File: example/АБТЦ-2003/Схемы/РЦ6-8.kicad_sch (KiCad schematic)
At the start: 32 parts

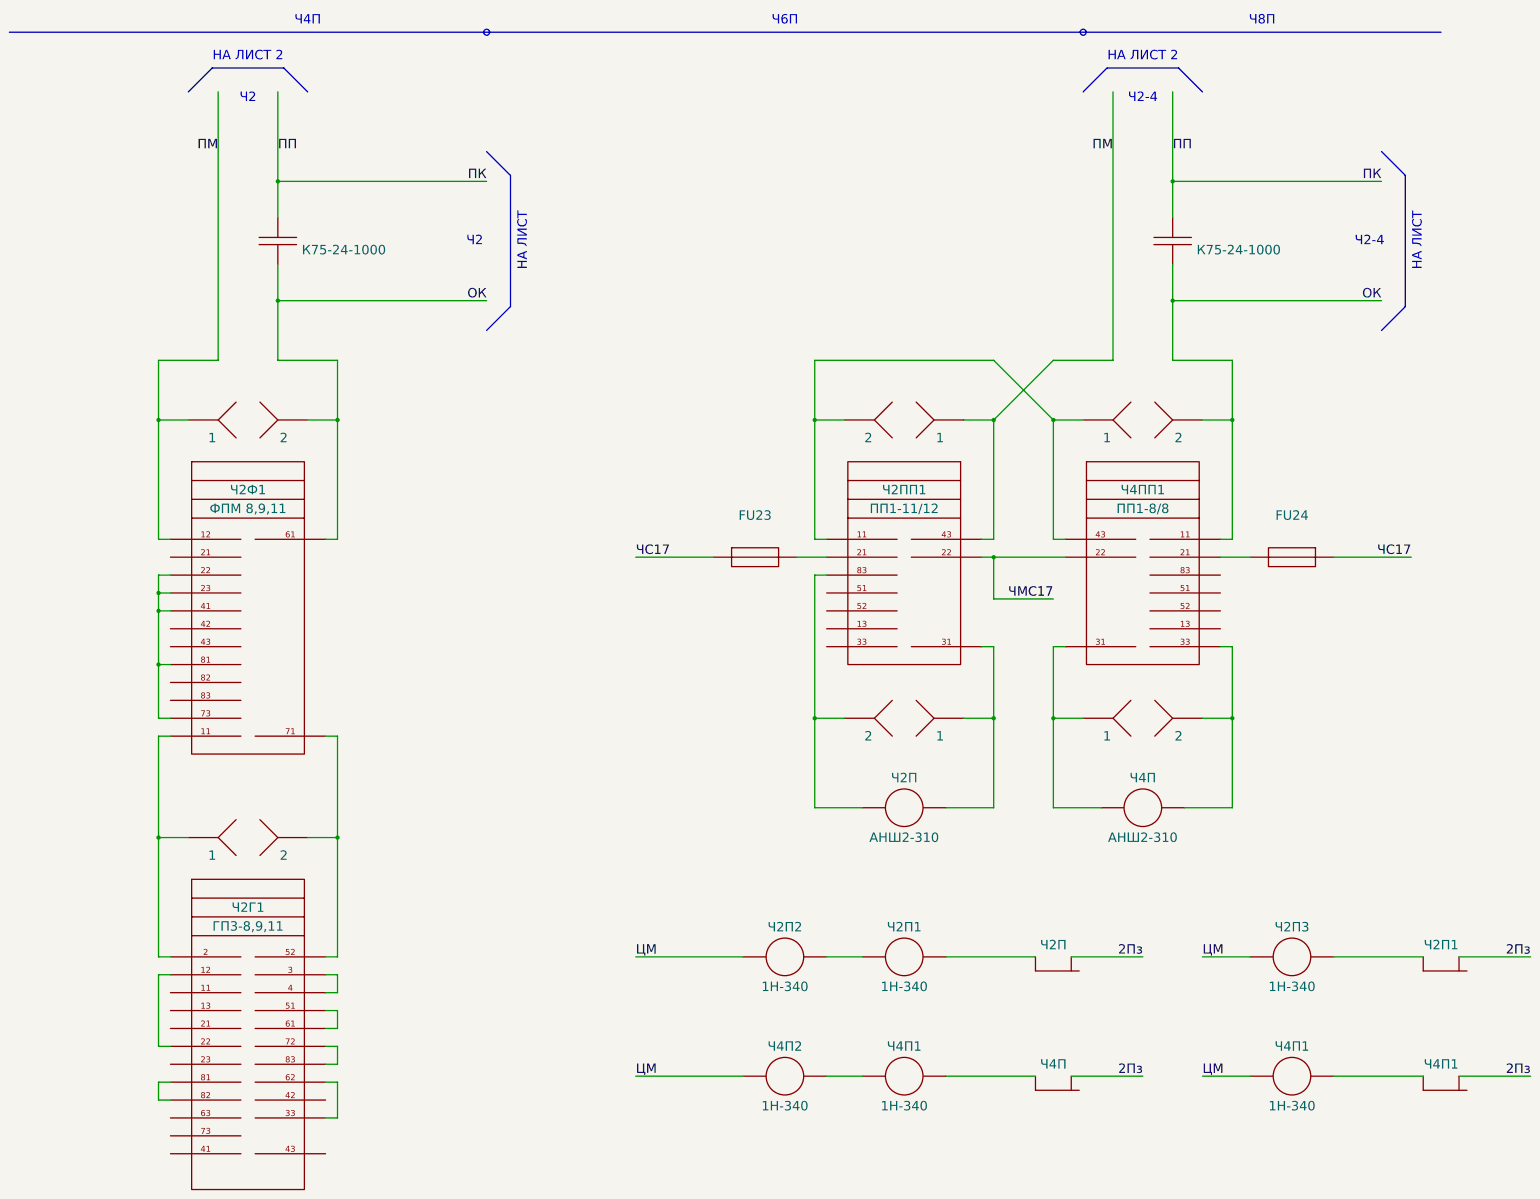
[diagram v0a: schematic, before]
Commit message: Шаблон АБТЦ обновлен
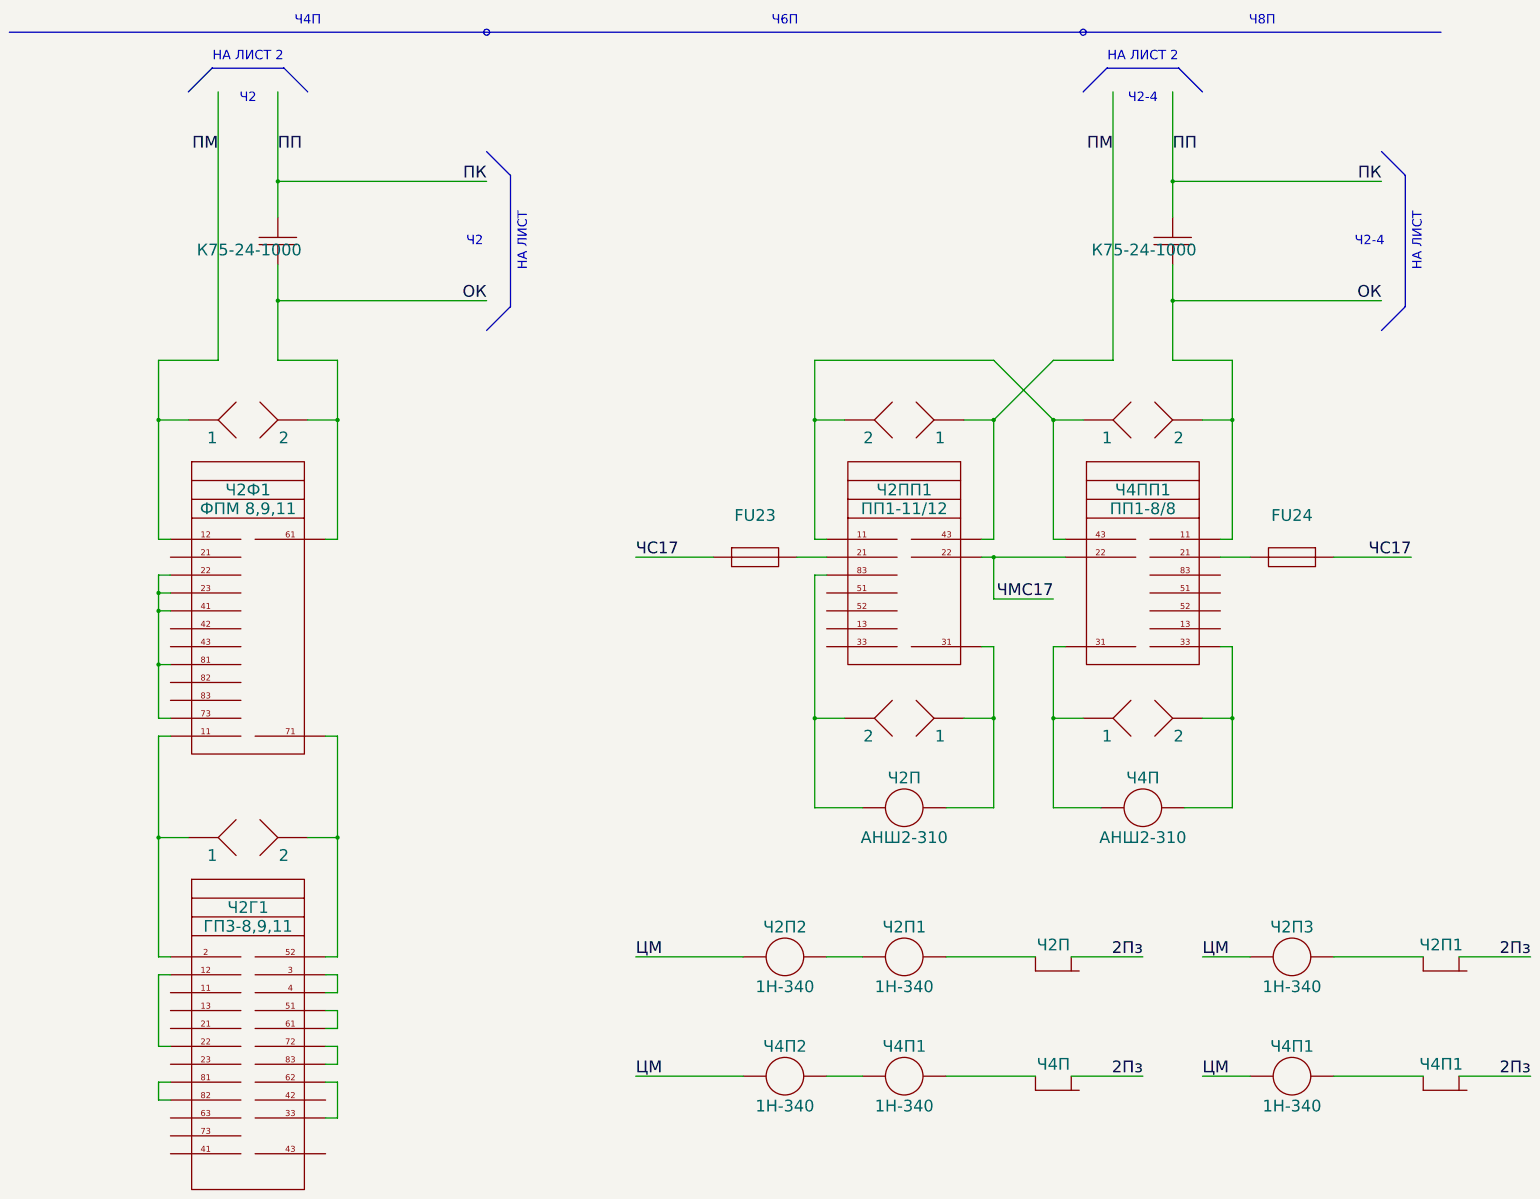
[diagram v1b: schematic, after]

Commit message: Обновление примера
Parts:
- Н11121, Н111211, Н11122, Н1113: symbol SCB_Relay:Контакт_нейтрального_якоря_НЗ -> SCB_Legacy:Контакт_нейтрального_якоря_НЗ_бн
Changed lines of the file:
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@@
 (kicad_sch
-	(version 20231120)
+	(version 20250114)
 	(generator "eeschema")
-	(generator_version "8.0")
+	(generator_version "9.0")
 	(paper "A3")
 	(title_block
@@
 		(comment 3 "Бузунова")
 	)
+	(circle
+		(center 152.4 31.75)
+		(radius 0.635)
+		(stroke
+			(width 0)
+			(type default)
+		)
+		(fill
+			(type color)
+			(color 0 0 0 0)
+		)
+	)
+	(circle
+		(center 279.4 31.75)
+		(radius 0.635)
+		(stroke
+			(width 0)
+			(type default)
+		)
+		(fill
+			(type color)
+			(color 0 0 0 0)
+		)
+	)
+	(text "Ч2"
+		(exclude_from_sim no)
+		(at 149.86 76.2 0)
+		(effects
+			(font
+				(size 2 2)
+			)
+		)
+	)
+	(text "НА ЛИСТ"
+		(exclude_from_sim no)
+		(at 350.52 76.2 90)
+		(effects
+			(font
+				(size 2 2)
+			)
+		)
+	)
+	(text "Ч2-4"
+		(exclude_from_sim no)
+		(at 292.1 45.72 0)
+		(effects
+			(font
+				(size 2 2)
+			)
+		)
+	)
+	(text "Ч2"
+		(exclude_from_sim no)
+		(at 101.6 45.72 0)
+		(effects
+			(font
+				(size 2 2)
+			)
+		)
+	)
+	(text "НА ЛИСТ 2"
+		(exclude_from_sim no)
+		(at 292.1 36.83 0)
+		(effects
+			(font
+				(size 2 2)
+			)
+		)
+	)
+	(text "Ч8П"
+		(exclude_from_sim no)
+		(at 317.5 29.21 0)
+		(effects
+			(font
+				(size 2 2)
+			)
+		)
+	)
+	(text "Ч2-4"
+		(exclude_from_sim no)
+		(at 340.36 76.2 0)
+		(effects
+			(font
+				(size 2 2)
+			)
+		)
+	)
+	(text "Ч6П"
+		(exclude_from_sim no)
+		(at 215.9 29.21 0)
+		(effects
+			(font
+				(size 2 2)
+			)
+		)
+	)
+	(text "НА ЛИСТ"
+		(exclude_from_sim no)
+		(at 160.02 76.2 90)
+		(effects
+			(font
+				(size 2 2)
+			)
+		)
+	)
+	(text "Ч4П"
+		(exclude_from_sim no)
+		(at 114.3 29.21 0)
+		(effects
+			(font
+				(size 2 2)
+			)
+		)
+	)
+	(text "НА ЛИСТ 2"
+		(exclude_from_sim no)
+		(at 101.6 36.83 0)
+		(effects
+			(font
+				(size 2 2)
+			)
+		)
+	)
 	(junction
 		(at 222.25 177.8)
@@
 		)
 	)
-	(circle
-		(center 152.4 31.75)
-		(radius 0.635)
-		(stroke
-			(width 0)
-			(type default)
-		)
-		(fill
-			(type color)
-			(color 0 0 0 0)
-		)
-	)
-	(circle
-		(center 279.4 31.75)
-		(radius 0.635)
-		(stroke
-			(width 0)
-			(type default)
-		)
-		(fill
-			(type color)
-			(color 0 0 0 0)
-		)
-	)
-	(text "Ч2"
-		(exclude_from_sim no)
-		(at 149.86 76.2 0)
-		(effects
-			(font
-				(size 2 2)
-			)
-		)
-	)
-	(text "НА ЛИСТ"
-		(exclude_from_sim no)
-		(at 350.52 76.2 90)
-		(effects
-			(font
-				(size 2 2)
-			)
-		)
-	)
-	(text "Ч2-4"
-		(exclude_from_sim no)
-		(at 292.1 45.72 0)
-		(effects
-			(font
-				(size 2 2)
-			)
-		)
-	)
-	(text "Ч2"
-		(exclude_from_sim no)
-		(at 101.6 45.72 0)
-		(effects
-			(font
-				(size 2 2)
-			)
-		)
-	)
-	(text "НА ЛИСТ 2"
-		(exclude_from_sim no)
-		(at 292.1 36.83 0)
-		(effects
-			(font
-				(size 2 2)
-			)
-		)
-	)
-	(text "Ч8П"
-		(exclude_from_sim no)
-		(at 317.5 29.21 0)
-		(effects
-			(font
-				(size 2 2)
-			)
-		)
-	)
-	(text "Ч2-4"
-		(exclude_from_sim no)
-		(at 340.36 76.2 0)
-		(effects
-			(font
-				(size 2 2)
-			)
-		)
-	)
-	(text "Ч6П"
-		(exclude_from_sim no)
-		(at 215.9 29.21 0)
-		(effects
-			(font
-				(size 2 2)
-			)
-		)
-	)
-	(text "НА ЛИСТ"
-		(exclude_from_sim no)
-		(at 160.02 76.2 90)
-		(effects
-			(font
-				(size 2 2)
-			)
-		)
-	)
-	(text "Ч4П"
-		(exclude_from_sim no)
-		(at 114.3 29.21 0)
-		(effects
-			(font
-				(size 2 2)
-			)
-		)
-	)
-	(text "НА ЛИСТ 2"
-		(exclude_from_sim no)
-		(at 101.6 36.83 0)
-		(effects
-			(font
-				(size 2 2)
-			)
-		)
-	)
 	(label "ЦМ"
 		(at 184.15 228.6 0)
@@
 	)
 	(symbol
-		(lib_id "SCB_Relay:Контакт_нейтрального_якоря_НЗ")
+		(lib_name "Контакт_нейтрального_якоря_НЗ_бн_1")
+		(lib_id "SCB_Legacy:Контакт_нейтрального_якоря_НЗ_бн")
 		(at 273.05 228.6 0)
 		(unit 3)
@@
 	)
 	(symbol
-		(lib_name "SCB_Relay:Контакт_нейтрального_якоря_НЗ")
-		(lib_id "SCB_Relay:Контакт_нейтрального_якоря_НЗ")
+		(lib_name "Контакт_нейтрального_якоря_НЗ_бн_3")
+		(lib_id "SCB_Legacy:Контакт_нейтрального_якоря_НЗ_бн")
 		(at 273.05 254 0)
 		(unit 3)
@@
 	)
 	(symbol
-		(lib_name "SCB_Relay:Контакт_нейтрального_якоря_НЗ")
-		(lib_id "SCB_Relay:Контакт_нейтрального_якоря_НЗ")
+		(lib_name "Контакт_нейтрального_якоря_НЗ_бн_2")
+		(lib_id "SCB_Legacy:Контакт_нейтрального_якоря_НЗ_бн")
 		(at 355.6 254 0)
 		(unit 3)
@@
 	)
 	(symbol
-		(lib_name "SCB_Relay:Контакт_нейтрального_якоря_НЗ")
-		(lib_id "SCB_Relay:Контакт_нейтрального_якоря_НЗ")
+		(lib_id "SCB_Legacy:Контакт_нейтрального_якоря_НЗ_бн")
 		(at 355.6 228.6 0)
 		(unit 3)
